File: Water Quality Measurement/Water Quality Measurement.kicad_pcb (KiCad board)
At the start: 2 copper layers, 166.6 x 73.9 mm, 14 parts, among them J1 pH Sensor, J2 OLED Screen, J3 MountingPin_IO1, J4 Conn_01x02_MountingPin, J5 MountingPin_IO46, J6 Voltage 9 ->5 regulator, Q1 2N2219, U1 LM7805_TO220

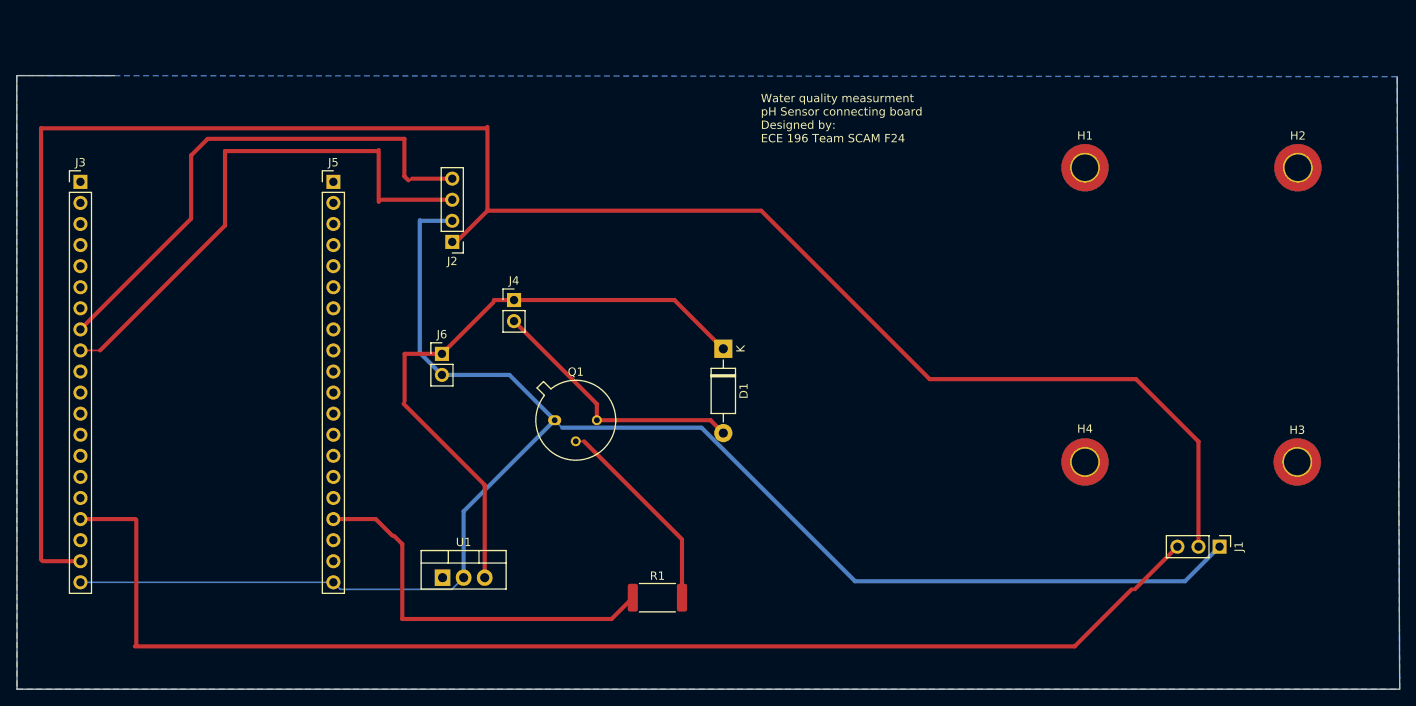
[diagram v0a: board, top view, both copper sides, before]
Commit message: Add files via upload
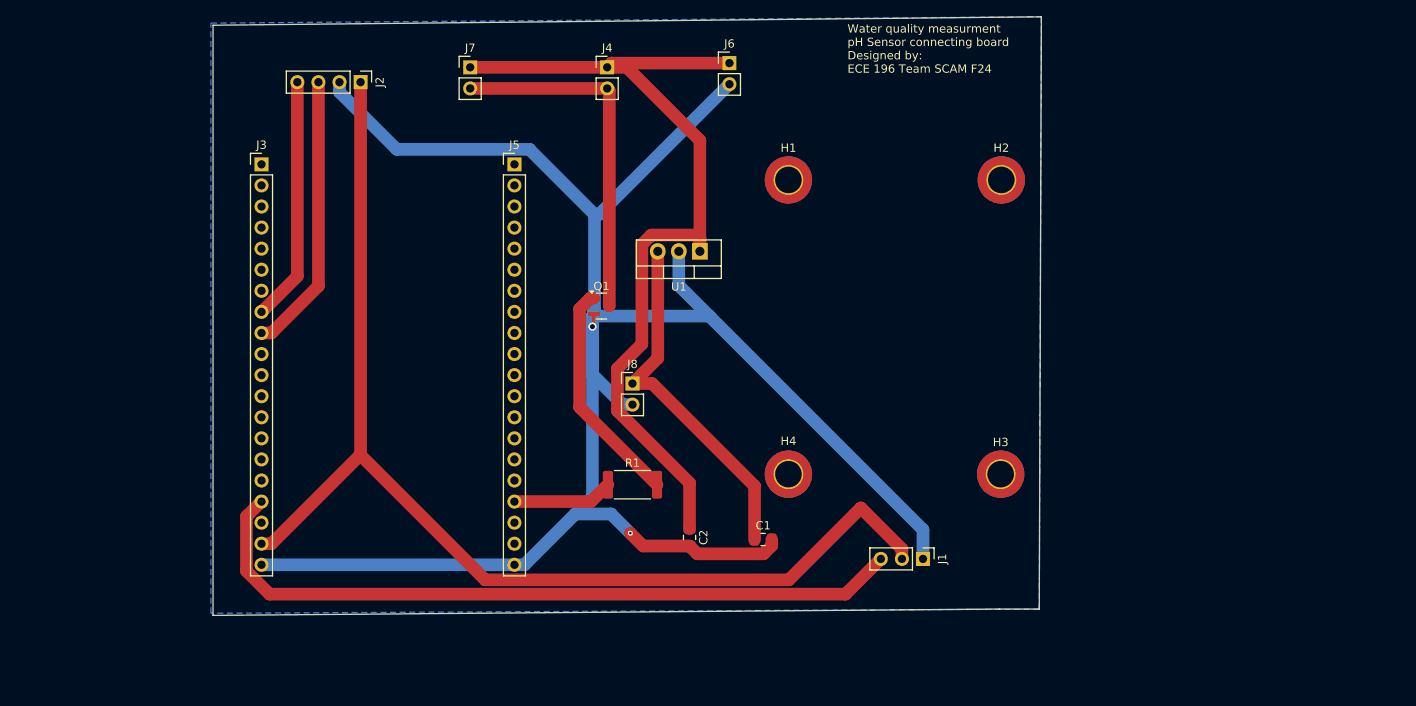
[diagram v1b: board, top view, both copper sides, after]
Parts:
- removed D1: 1N4007, Diode_THT:D_DO-41_SOD81_P10.16mm_Horizontal
- added C1: 0.1u, Capacitor_SMD:C_0805_2012Metric_Pad1.18x1.45mm_HandSolder, F.Cu at (157.5, 109.7)
- added C2: 0.22u, Capacitor_SMD:C_0805_2012Metric_Pad1.18x1.45mm_HandSolder, F.Cu at (148.6, 109.5)
- added J7: Conn_01x02_MountingPin, Connector_PinHeader_2.54mm:PinHeader_1x02_P2.54mm_Vertical, F.Cu at (122.2, 52.8)
- added J8: 9V Battery Enclosure, Connector_PinHeader_2.54mm:PinHeader_1x02_P2.54mm_Vertical, F.Cu at (141.7, 90.9)
- J6: value Voltage 9 ->5 regulator -> 9V Battery Enclosure
- Q1: value 2N2219 -> PMV15UNEAR; footprint Package_TO_SOT_THT:TO-39-3 -> Package_TO_SOT_SMD:SOT-23
- R1: value R_US -> 1k
- moved U1 50.1 mm to (149.9, 75.0), turned to 180 degrees
- moved J6 49.3 mm to (153.4, 52.3)
- moved H1 35.8 mm to (160.5, 66.4)
- moved H2 35.8 mm to (186.2, 66.4)
- moved H3 35.8 mm to (186.1, 101.9)
- moved H4 35.8 mm to (160.5, 101.9)
- moved J1 35.8 mm to (176.7, 112.1)
- moved J4 30.2 mm to (138.7, 52.8)
- moved J2 22.2 mm to (109.0, 54.6), turned to -90 degrees
- moved J3 21.9 mm to (97.0, 64.5)
- moved J5 21.9 mm to (127.5, 64.5)
- moved Q1 14.9 mm to (138.0, 81.6)
- moved R1 13.9 mm to (141.7, 103.1)
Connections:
- J4 pad 1: /Vbatt -> Net-(J4-Pin_1)
- J5 pad 1: (no net) -> unconnected-(J5-Pin_1-Pad1)
- J5 pad 10: (no net) -> unconnected-(J5-Pin_10-Pad10)
- J5 pad 11: (no net) -> unconnected-(J5-Pin_11-Pad11)
- J5 pad 12: (no net) -> unconnected-(J5-Pin_12-Pad12)
- J5 pad 13: (no net) -> unconnected-(J5-Pin_13-Pad13)
- J5 pad 14: (no net) -> unconnected-(J5-Pin_14-Pad14)
- J5 pad 15: (no net) -> unconnected-(J5-Pin_15-Pad15)
- J5 pad 16: (no net) -> unconnected-(J5-Pin_16-Pad16)
- J5 pad 18: (no net) -> unconnected-(J5-Pin_18-Pad18)
- J5 pad 19: (no net) -> unconnected-(J5-Pin_19-Pad19)
- J5 pad 2: (no net) -> unconnected-(J5-Pin_2-Pad2)
- J5 pad 3: (no net) -> unconnected-(J5-Pin_3-Pad3)
- J5 pad 4: (no net) -> unconnected-(J5-Pin_4-Pad4)
- J5 pad 5: (no net) -> unconnected-(J5-Pin_5-Pad5)
- J5 pad 6: (no net) -> unconnected-(J5-Pin_6-Pad6)
- J5 pad 7: (no net) -> unconnected-(J5-Pin_7-Pad7)
- J5 pad 8: (no net) -> unconnected-(J5-Pin_8-Pad8)
- J5 pad 9: (no net) -> unconnected-(J5-Pin_9-Pad9)
- J6 pad 1: /Vbatt -> Net-(J4-Pin_1)
- Q1 pad 1: GND -> Net-(Q1-G)
- Q1 pad 2: Net-(Q1-B) -> GND
- R1 pad 2: Net-(Q1-B) -> Net-(Q1-G)
- U1 pad 1: /9V enclosure -> Net-(J4-Pin_1)
- U1 pad 3: /Vbatt -> Net-(J8-Pin_1)
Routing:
- net Net-(J4-Pin_1): track 0.00 -> 108.0 mm
- net /3.3: track 236.5 -> 139.6 mm
- net /Vbatt: track 74.7 -> 0.00 mm
- net pH sen. input: track 152.7 -> 88.5 mm
- net Net-(J8-Pin_1): track 0.00 -> 43.5 mm
- net GND: track 200.1 -> 243.4 mm, vias 0 -> 2
- net /IO26: track 47.4 -> 12.1 mm
- net SDA: track 63.6 -> 29.5 mm
- net SCL: track 66.5 -> 33.8 mm
- net Net-(Q1-G): track 0.00 -> 27.3 mm
- net Net-(Q1-B): track 24.7 -> 0.00 mm
- net Net-(J4-Pin_2): track 32.0 -> 42.8 mm
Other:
- board size 166.6 x 73.9 mm -> 99.8 x 72.1 mm
